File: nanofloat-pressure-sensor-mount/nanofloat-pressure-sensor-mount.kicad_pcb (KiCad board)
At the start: 2 copper layers, 5.8 x 6.4 mm, 2 parts, among them J1 Conn_01x04_Pin

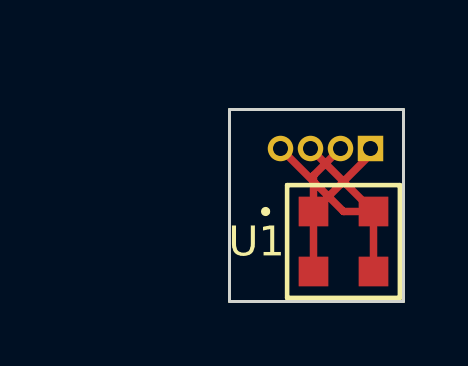
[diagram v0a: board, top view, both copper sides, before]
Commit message: Updating KiCAD project files
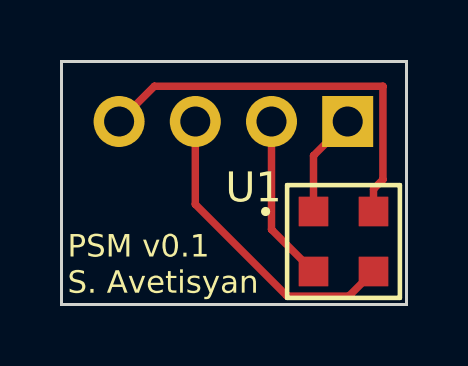
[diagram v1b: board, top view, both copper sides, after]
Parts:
- J1: footprint Connector_PinHeader_1.00mm:PinHeader_1x04_P1.00mm_Vertical -> Connector_PinHeader_2.54mm:PinHeader_1x04_P2.54mm_Vertical
- moved J1 1.18 mm to (148.1, 88.0)
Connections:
- J1 pad 2: Net-(J1-Pin_1) -> Net-(J1-Pin_2)
- J1 pad 3: Net-(J1-Pin_1) -> Net-(J1-Pin_3)
- J1 pad 4: Net-(J1-Pin_1) -> Net-(J1-Pin_4)
- U1 pad 2: Net-(J1-Pin_1) -> Net-(J1-Pin_2)
- U1 pad 3: Net-(J1-Pin_1) -> Net-(J1-Pin_3)
- U1 pad 4: Net-(J1-Pin_1) -> Net-(J1-Pin_4)
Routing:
- net Net-(J1-Pin_4): track 0.00 -> 13.6 mm
- net Net-(J1-Pin_1): track 16.3 -> 3.47 mm
- net Net-(J1-Pin_3): track 0.00 -> 10.3 mm
- net Net-(J1-Pin_2): track 0.00 -> 5.58 mm
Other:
- board size 5.8 x 6.4 mm -> 11.5 x 8.1 mm
- board text added: "PSM v0.1 S. Avetisyan"
